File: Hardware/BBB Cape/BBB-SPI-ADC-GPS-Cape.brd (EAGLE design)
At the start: 100 x 80 mm, 6 parts

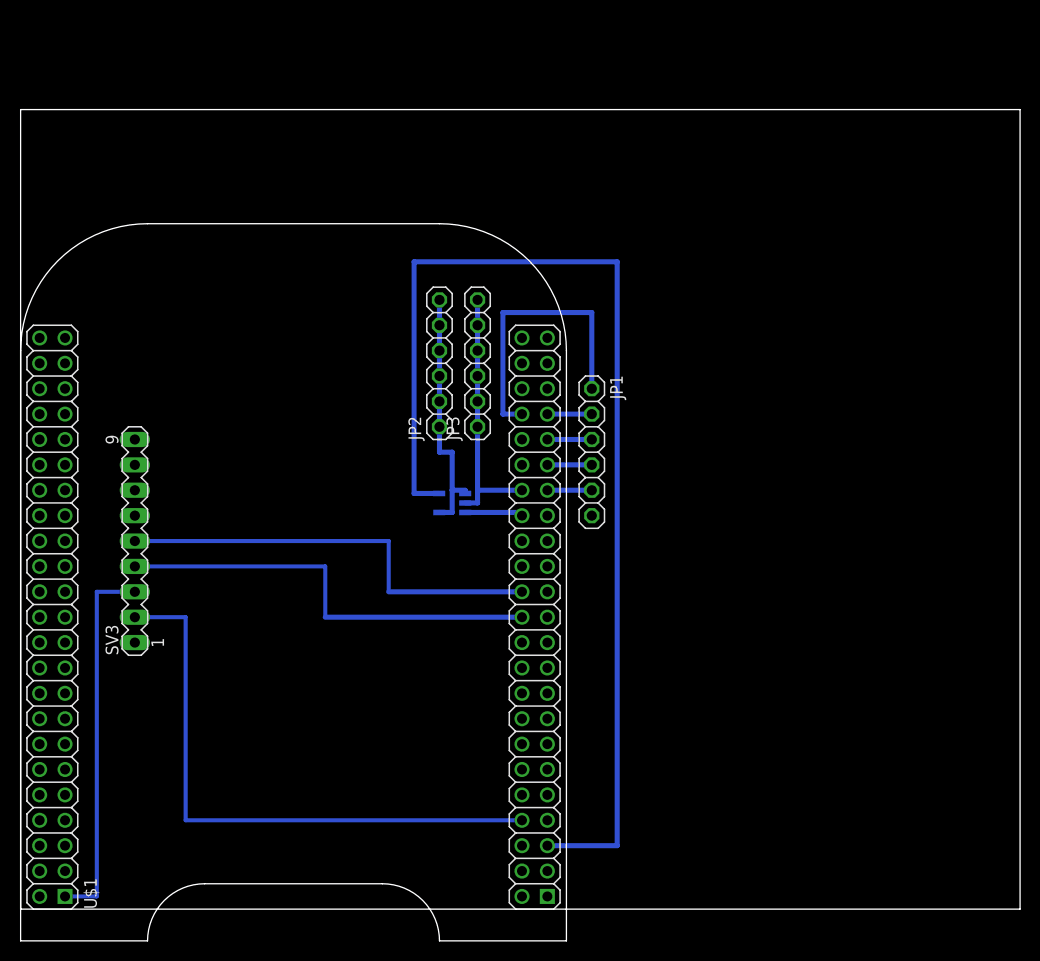
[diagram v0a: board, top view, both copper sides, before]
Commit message: working version of the adc/gps cape
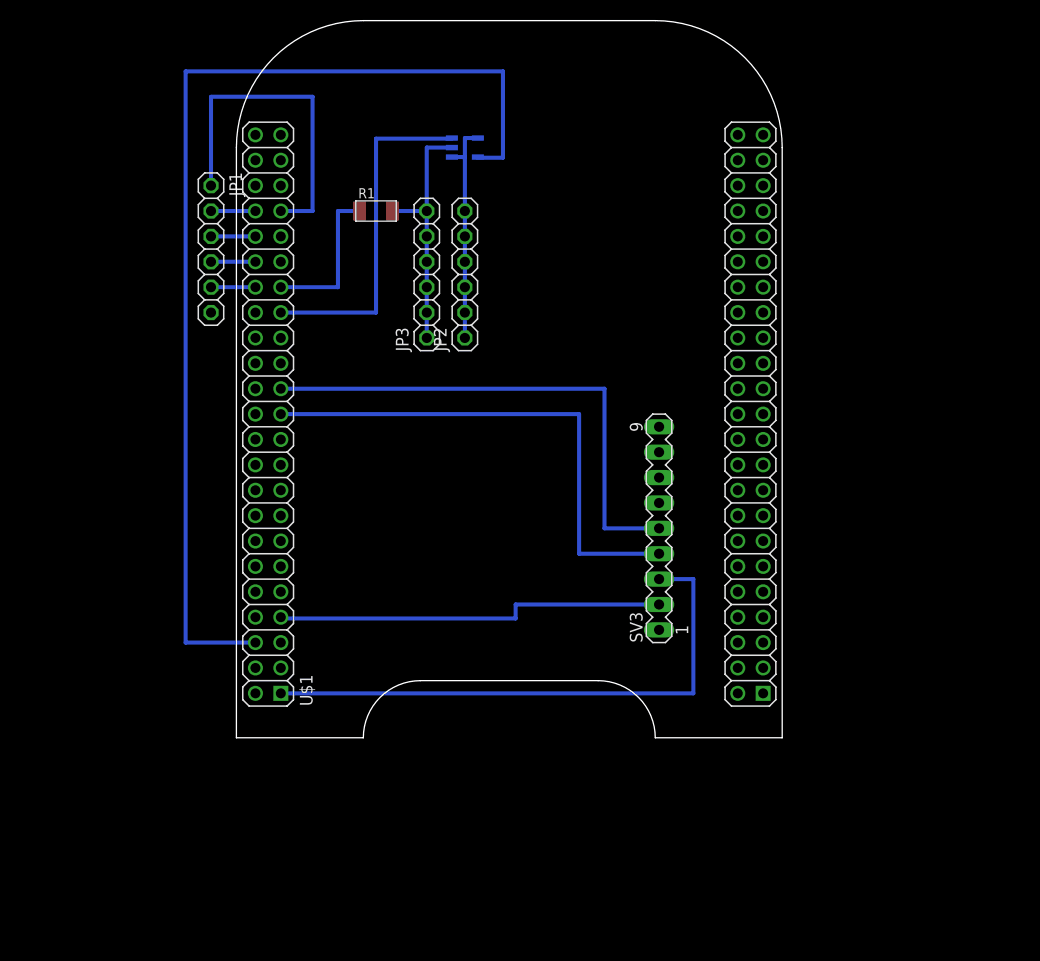
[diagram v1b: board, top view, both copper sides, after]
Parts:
- removed U$4: OPA344, SparkFun-AnalogIC:SOT23-5
- added LMP_OP-AMP: OPA344, SparkFun-AnalogIC:SOT23-5
- added R1: (no value), fab:R1206FAB
- moved SV3 52.5 mm to (63.9, 38.1)
- moved JP1 43.2 mm to (19.1, 66.0)
- moved U$1 29.6 mm to (21.6, 2.54)
- moved JP3 10.2 mm to (40.6, 63.5)
- moved JP2 9.25 mm to (44.5, 63.5)
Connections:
- net SYS_5V renamed N$1
- net GNDA_ADC: now also LMP_OP-AMP.2; no longer U$4.2
- net N$2: now also LMP_OP-AMP.1, LMP_OP-AMP.4; no longer U$4.1, U$4.4
- net VDD_5V: now also LMP_OP-AMP.5; no longer U$4.5
- net VDD_ADC: now also LMP_OP-AMP.3; no longer U$4.3
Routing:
- net VDD_5V: track 111.4 -> 0.00 mm
- net N$7: track 0.00 -> 107.1 mm
- net N$4: track 0.00 -> 51.7 mm
- net N$3: track 0.00 -> 51.7 mm
- net TX-B: track 43.8 -> 0.00 mm
- net RX-B: track 43.8 -> 0.00 mm
- net N$5: track 0.00 -> 34.5 mm
- net N$1: track 59.1 -> 39.1 mm
- net GND: track 37.5 -> 56.1 mm
- net N$6: track 0.00 -> 15.9 mm
- net VDD_ADC: track 6.00 -> 0.00 mm
- net AIN1: track 28.6 -> 33.7 mm
- net N$2: track 25.5 -> 22.6 mm
- net GNDA_ADC: track 26.0 -> 25.4 mm
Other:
- board size 100 x 80 mm -> 54.6 x 71.8 mm
